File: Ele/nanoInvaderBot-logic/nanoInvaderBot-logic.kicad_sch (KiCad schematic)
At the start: 18 parts, among them J3 1746142-1, J4 Conn_01x20, P1 USB_C_Plug_USB2.0, U4 BQ25170DSGR, U5 TLV61048DBVT

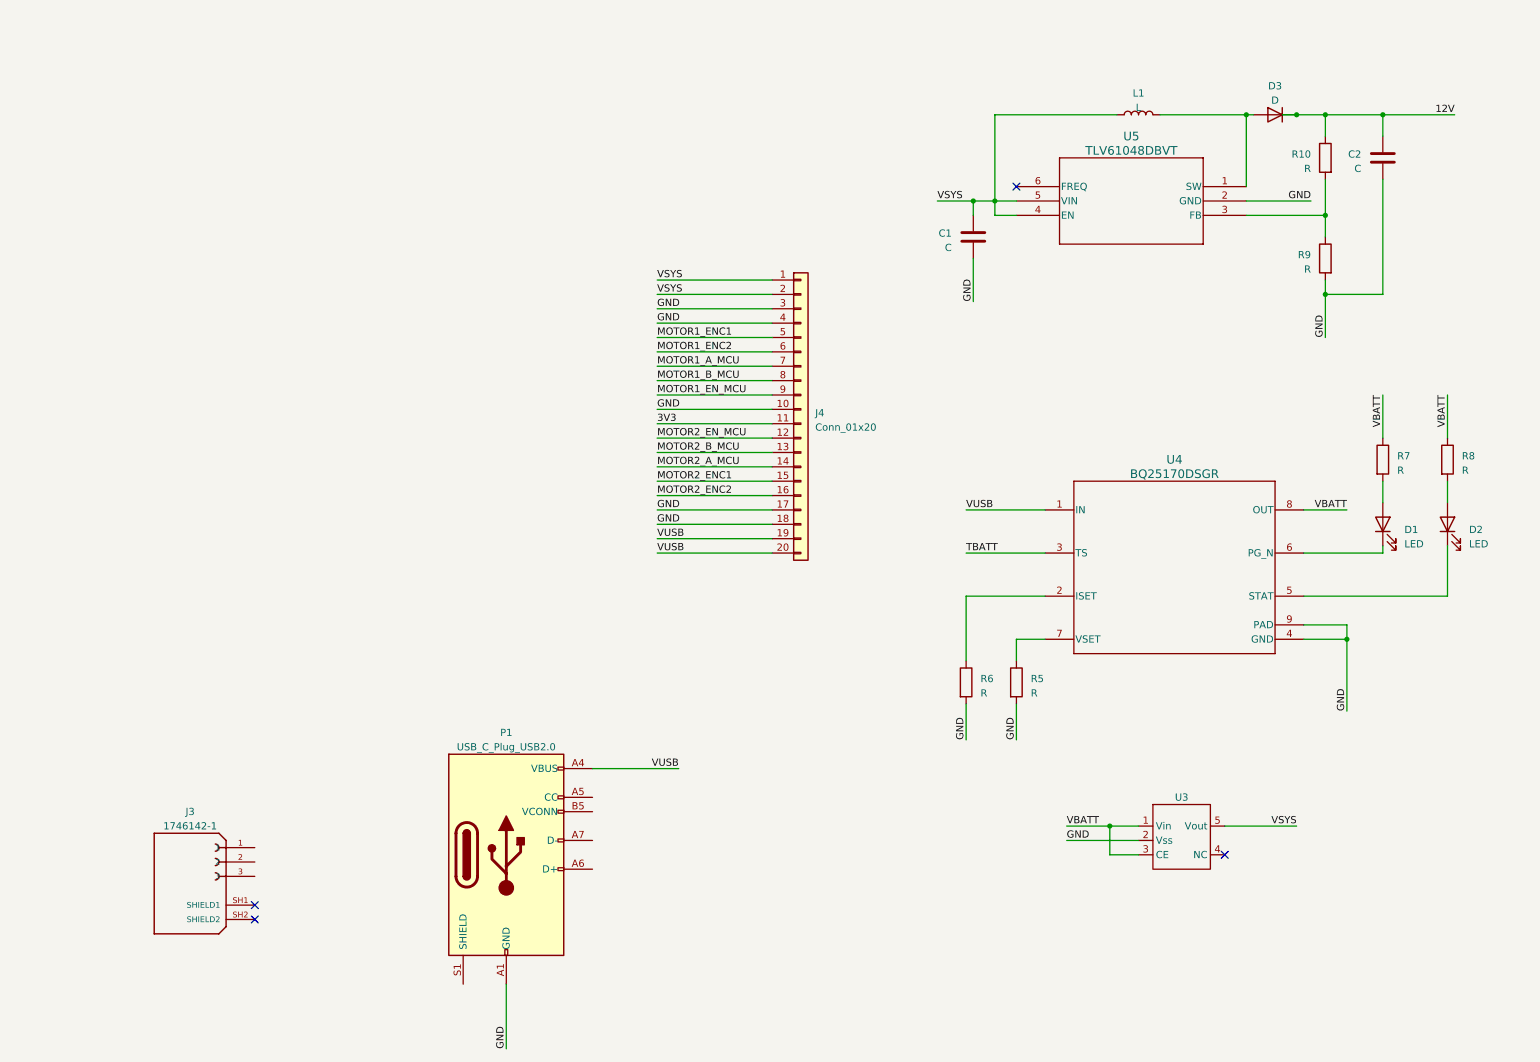
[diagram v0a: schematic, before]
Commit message: Intermediate state after v23.10
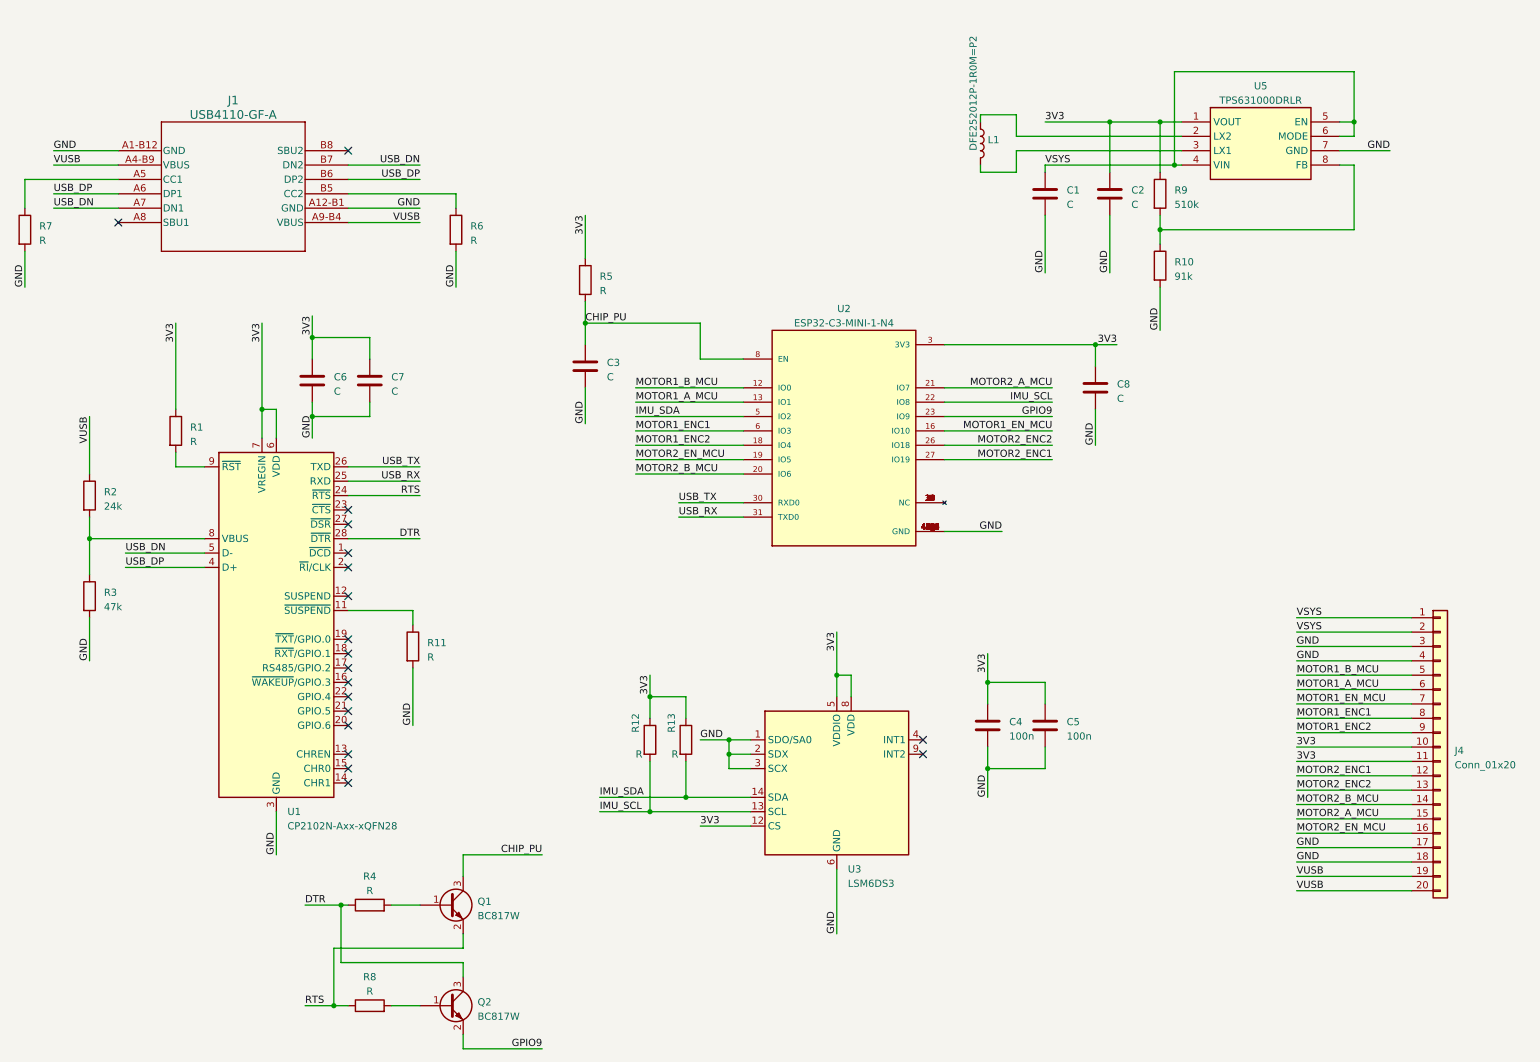
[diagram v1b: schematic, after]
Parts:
- removed D1, D2: LED, LED_SMD:LED_0603_1608Metric, symbol Device:LED
- removed D3: D, symbol Device:D
- removed J3: 1746142-1, footprints:TE_1746142-1, symbol 1746142-1:1746142-1
- removed P1: USB_C_Plug_USB2.0, Connector_USB:USB_C_Receptacle_GCT_USB4135-GF-A_6P_TopMnt_Horizontal, symbol Connector:USB_C_Plug_USB2.0
- removed U3: ~, Package_TO_SOT_SMD:SOT-23-5, symbol XC8111:XC8111-MR-G
- removed U4: BQ25170DSGR, footprints:BQ25170DSGR_NV, symbol BQ25170DSGR:BQ25170DSGR
- removed U5: TLV61048DBVT, SOT23-6_DBV_TEX, symbol TLV61048DBVT:TLV61048DBVT
- added C3: C, Capacitor_SMD:C_0603_1608Metric, symbol Device:C
- added C4, C5: 100n, Capacitor_SMD:C_0603_1608Metric, symbol Device:C
- added C6, C7, C8: C, Capacitor_SMD:C_0805_2012Metric, symbol Device:C
- added J1: USB4110-GF-A, footprints:USB4110-GF-A_GCT, symbol USB4110-GF-A:USB4110-GF-A
- added Q1, Q2: BC817W, Package_TO_SOT_SMD:SOT-323_SC-70, symbol Transistor_BJT:BC817W
- added R1, R11, R12, R13, R4: R, Resistor_SMD:R_0402_1005Metric, symbol Device:R
- added R2: 24k, Resistor_SMD:R_0402_1005Metric, symbol Device:R
- added R3: 47k, Resistor_SMD:R_0402_1005Metric, symbol Device:R
- added U1: CP2102N-Axx-xQFN28, Package_DFN_QFN:QFN-28-1EP_5x5mm_P0.5mm_EP3.35x3.35mm, symbol Interface_USB:CP2102N-Axx-xQFN28
- added U2: ESP32-C3-MINI-1-N4, footprints:XCVR_ESP32-C3-MINI-1-N4, symbol ESP32-C3-MINI-1-N4:ESP32-C3-MINI-1-N4
- added U3: LSM6DS3, Package_LGA:LGA-14_3x2.5mm_P0.5mm_LayoutBorder3x4y, symbol Sensor_Motion:LSM6DS3
- added U5: TPS631000DRLR, footprints:SOTFL50P160X60-8N, symbol TPS631000DRLR:TPS631000DRLR
- C1, C2: footprint (none) -> Capacitor_SMD:C_0805_2012Metric
- L1: value L -> DFE252012P-1R0M=P2; footprint (none) -> Inductor_SMD:L_2512_6332Metric
- R10: value R -> 91k; footprint (none) -> Resistor_SMD:R_0402_1005Metric
- R5, R6, R7, R8: footprint Resistor_SMD:R_0603_1608Metric -> Resistor_SMD:R_0402_1005Metric
- R9: value R -> 510k; footprint (none) -> Resistor_SMD:R_0402_1005Metric
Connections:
- net 3V3: now also C2.1, J4.10 (Pin_10), R5.1, R9.1, C4.1, C5.1, C6.2, C7.2, C8.2, R1.1, R12.1, R13.1, U1.6 (VDD), U1.7 (VREGIN), U2.3 (3V3), U3.12 (CS), U3.5 (VDDIO), U3.8 (VDD), U5.1 (VOUT)
- net GND: now also R10.2, R7.2, C3.2, C4.2, C5.2, C6.1, C7.1, C8.1, J1.A1-B12 (GND), J1.A12-B1 (GND), R11.2, R3.2, U1.29 (GND), U1.3 (GND), U2.1 (GND), U2.11 (GND), U2.14 (GND), U2.2 (GND), U2.36 (GND), U2.37 (GND), U2.38 (GND), U2.39 (GND), U2.40 (GND), U2.41 (GND), U2.42 (GND), U2.43 (GND), U2.44 (GND), U2.45 (GND), U2.46 (GND), U2.47 (GND), U2.48 (GND), U2.49_1 (GND), U2.49_2 (GND), U2.49_3 (GND), U2.49_4 (GND), U2.49_5 (GND), U2.49_6 (GND), U2.49_7 (GND), U2.49_8 (GND), U2.49_9 (GND), U2.50 (GND), U2.51 (GND), U2.52 (GND), U2.53 (GND), U3.1 (SDO/SA0), U3.2 (SDX), U3.3 (SCX), U3.6 (GND), U3.7 (GND), U5.7 (GND); no longer J4.10 (Pin_10), R5.2, R9.2
- net MOTOR1_A_MCU: now also J4.6 (Pin_6), U2.13 (IO1); no longer J4.7 (Pin_7)
- net MOTOR1_B_MCU: now also J4.5 (Pin_5), U2.12 (IO0); no longer J4.8 (Pin_8)
- net MOTOR1_ENC1: now also J4.8 (Pin_8), U2.6 (IO3); no longer J4.5 (Pin_5)
- net MOTOR1_ENC2: now also J4.9 (Pin_9), U2.18 (IO4); no longer J4.6 (Pin_6)
- net MOTOR1_EN_MCU: now also J4.7 (Pin_7), U2.16 (IO10); no longer J4.9 (Pin_9)
- net MOTOR2_A_MCU: now also J4.15 (Pin_15), U2.21 (IO7); no longer J4.14 (Pin_14)
- net MOTOR2_B_MCU: now also J4.14 (Pin_14), U2.20 (IO6); no longer J4.13 (Pin_13)
- net MOTOR2_ENC1: now also J4.12 (Pin_12), U2.27 (IO19); no longer J4.15 (Pin_15)
- net MOTOR2_ENC2: now also J4.13 (Pin_13), U2.26 (IO18); no longer J4.16 (Pin_16)
- net MOTOR2_EN_MCU: now also J4.16 (Pin_16), U2.19 (IO5); no longer J4.12 (Pin_12)
- net VSYS: now also U5.4 (VIN), U5.5 (EN), U5.6 (MODE); no longer L1.2
- net VUSB: now also J1.A4-B9 (VBUS), J1.A9-B4 (VBUS), R2.1
- net at R6.1: now also J1.B5 (CC2)
- net at R8.2: now also Q2.1 (B)
- net at L1.1: now also U5.2 (LX2)
- net 12V: no longer names the net of R10.1
- net 12V: now also R9.2, U5.8 (FB); no longer C2.1
- net VBATT: no longer names the net of R7.1
- net VBATT: now also J1.A5 (CC1); no longer R8.1
- new net: R11.1, U1.11 (~{SUSPEND})
- new net: R2.2, R3.1, U1.8 (VBUS)
- new net: L1.2, U5.3 (LX1)
- new net: R1.2, U1.9 (~{RST})
- new net: U2.10 (NC), U2.15 (NC), U2.17 (NC), U2.24 (NC), U2.25 (NC), U2.28 (NC), U2.29 (NC), U2.32 (NC), U2.33 (NC), U2.34 (NC), U2.35 (NC), U2.4 (NC), U2.7 (NC), U2.9 (NC)
- new net: Q1.1 (B), R4.2
- new net CHIP_PU: C3.1, Q1.3 (C), R5.2, U2.8 (EN)
- new net DTR: Q2.3 (C), R4.1, U1.28 (~{DTR})
- new net GPIO9: Q2.2 (E), U2.23 (IO9)
- new net IMU_SCL: R12.2, U2.22 (IO8), U3.13 (SCL)
- new net IMU_SDA: R13.2, U2.5 (IO2), U3.14 (SDA)
- new net RTS: Q1.2 (E), R8.1, U1.24 (~{RTS})
- new net USB_DN: J1.A7 (DN1), J1.B7 (DN2), U1.5 (D-)
- new net USB_DP: J1.A6 (DP1), J1.B6 (DP2), U1.4 (D+)
- new net USB_RX: U1.25 (RXD), U2.31 (TXD0)
- new net USB_TX: U1.26 (TXD), U2.30 (RXD0)
- no-connect marks 4 -> 19
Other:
- moved on the sheet: J4
